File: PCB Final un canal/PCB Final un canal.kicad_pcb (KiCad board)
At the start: 2 copper layers, 60 x 50 mm, 32 parts, among them J1 Conn_01x02, J2 Conn_01x03, J3 Conn_01x02, U1 LM324, U2 AD620, U3 LM324

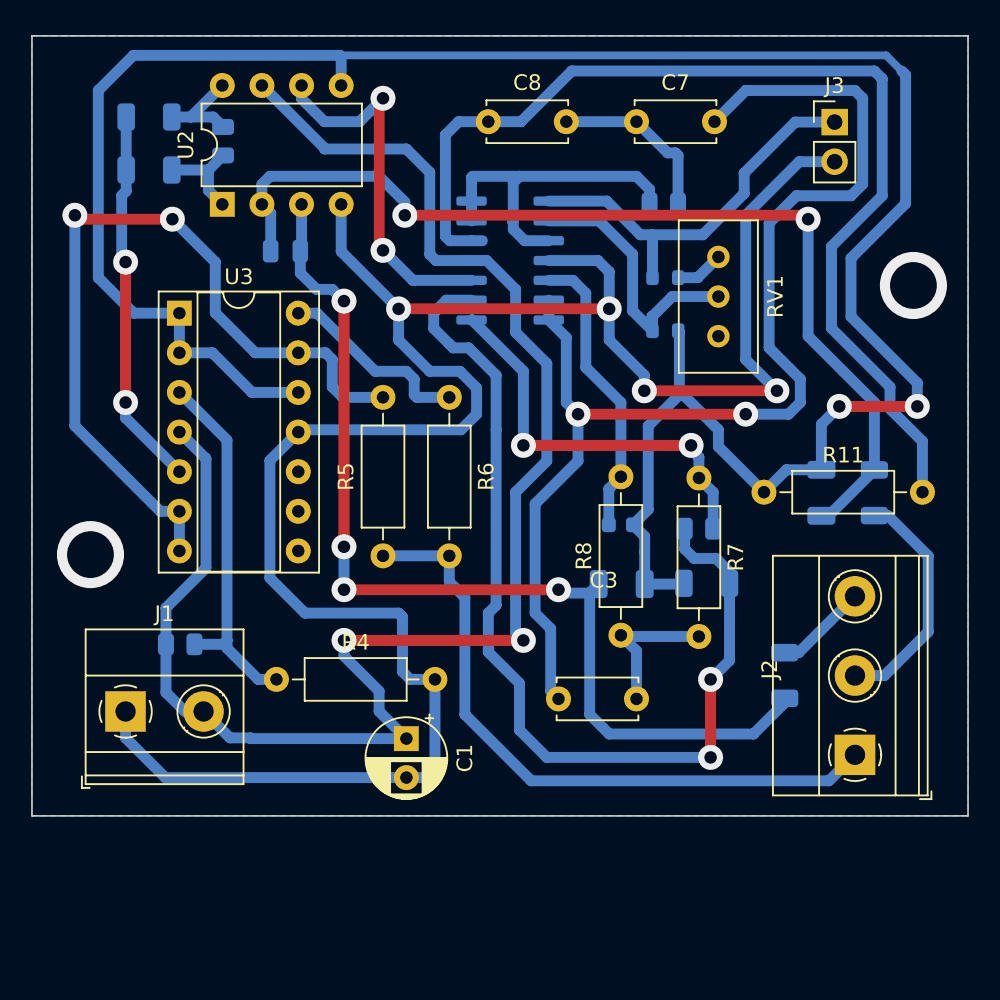
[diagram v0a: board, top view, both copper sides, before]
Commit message: Trabajo final completo
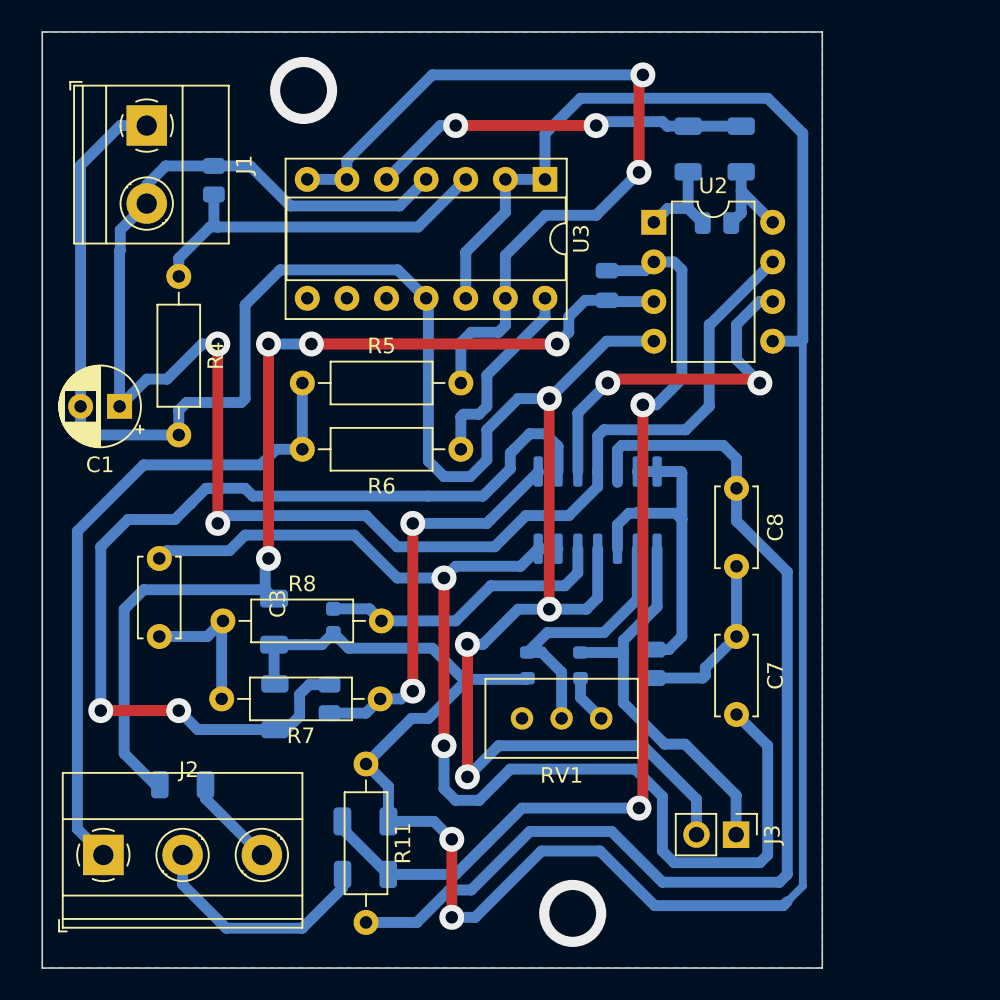
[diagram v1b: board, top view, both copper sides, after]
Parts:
- moved J2 48.6 mm to (27.3, 71.5), turned to 0 degrees
- moved J3 46.1 mm to (67.9, 70.2), turned to -90 degrees
- moved R9 40.8 mm to (44.1, 72.8), turned to 0 degrees
- moved R10 39.2 mm to (32.4, 67.0), turned to 180 degrees
- moved R2 38.0 mm to (68.2, 26.2), turned to -90 degrees
- moved J1 37.6 mm to (30.1, 24.8), turned to -90 degrees
- moved C5 36.0 mm to (44.1, 69.3), turned to 0 degrees
- moved R1 34.6 mm to (64.8, 26.2), turned to 90 degrees
- moved C7 33.6 mm to (67.9, 57.5), turned to -90 degrees
- moved R13 32.1 mm to (66.7, 31.0), turned to 180 degrees
- moved R11 30.9 mm to (44.2, 65.7), turned to -90 degrees
- moved R3 29.8 mm to (34.4, 28.2), turned to -90 degrees
- moved R12 29.5 mm to (62.7, 59.2), turned to -90 degrees
- moved R15 28.8 mm to (38.3, 62.0), turned to 90 degrees
- moved C8 28.4 mm to (67.9, 48.0), turned to -90 degrees
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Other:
- board size 60 x 50 mm -> 50 x 60 mm
